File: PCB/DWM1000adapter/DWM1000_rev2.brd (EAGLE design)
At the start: 33.1 x 27.1 mm, 9 parts, among them IC1 DWM1000

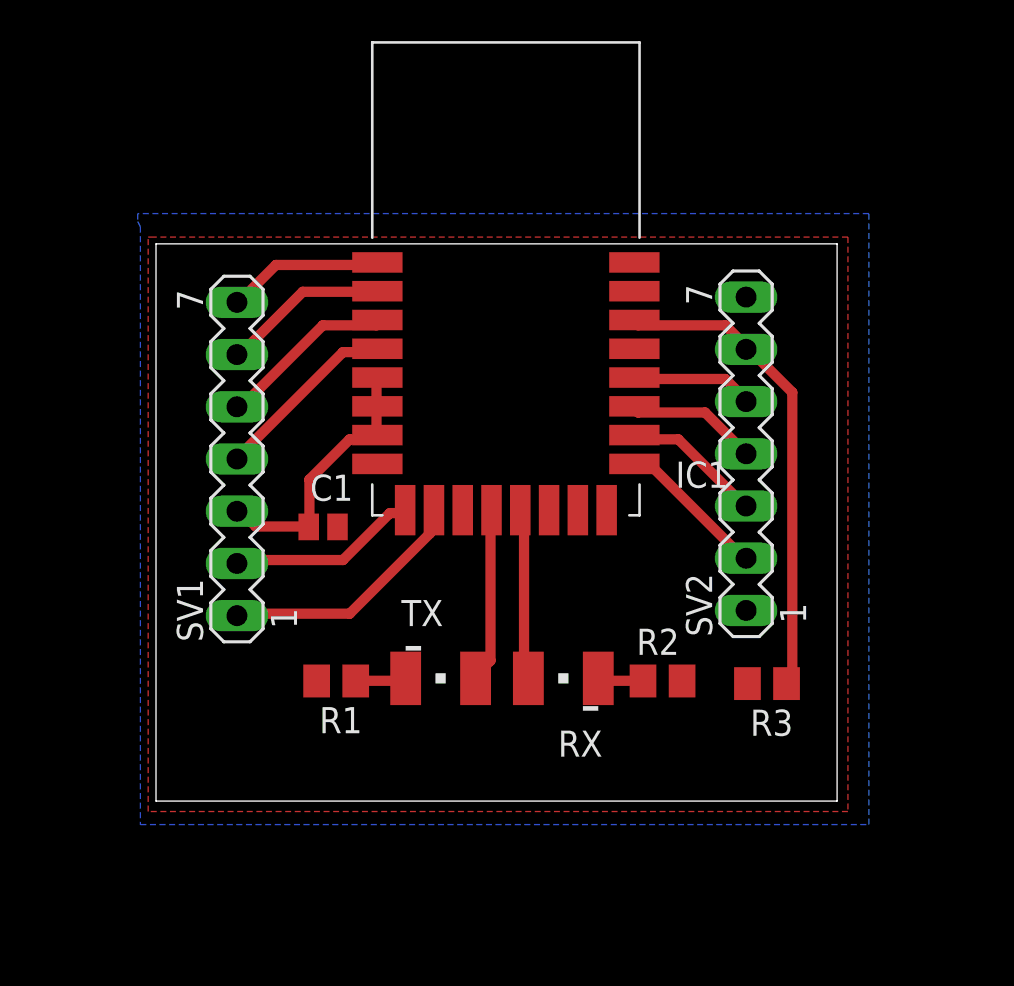
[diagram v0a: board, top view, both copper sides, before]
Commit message: knas
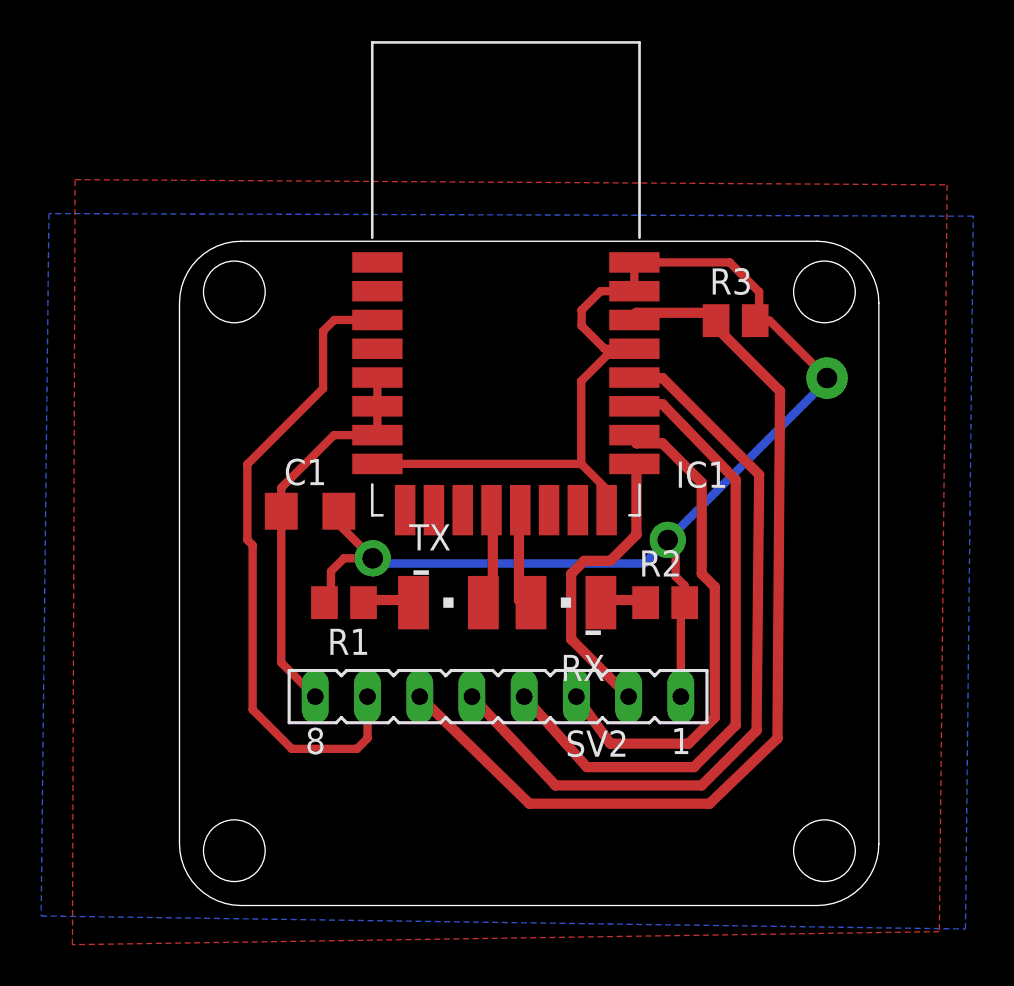
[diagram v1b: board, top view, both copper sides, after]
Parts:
- removed SV1: (no value), con-lstb:MA07-1
- C1: device eagle-ltspice:C0504 -> eagle-ltspice:C1206
- SV2: device con-lstb:MA07-1 -> con-lsta:FE08
- moved R3 17.7 mm to (31.5, 25.0), turned to 0 degrees
- moved SV2 16.9 mm to (19.9, 6.73), turned to 180 degrees
- moved R1 3.83 mm to (12.4, 11.3)
- moved R2 3.81 mm to (28.1, 11.3)
- moved TX 3.70 mm to (17.5, 11.3)
- moved RX 3.69 mm to (23.2, 11.3)
- moved C1 0.99 mm to (10.8, 15.7)
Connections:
- net 3.3: now also SV2.8; no longer SV1.3
- net EXT: no longer SV1.7
- net GND: no longer SV2.7
- net RST: now also SV2.7; no longer SV1.5
- net SPIPHA: no longer SV1.2
- net SPIPOL: no longer SV1.1
- net SYNC: no longer SV1.4
- net WAKE: no longer SV1.6
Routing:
- net GND: track 0.00 -> 82.9 mm, vias 0 -> 3
- net CLK: track 5.94 -> 37.3 mm
- net MISO: track 6.44 -> 31.1 mm
- net IRQ: track 23.6 -> 47.0 mm
- net RST: track 8.68 -> 31.5 mm
- net MOSI: track 6.88 -> 24.5 mm
- net SPIPOL: track 12.2 -> 0.00 mm
- net SPIPHA: track 9.25 -> 0.00 mm
- net SYNC: track 9.12 -> 0.00 mm
- net WAKE: track 8.08 -> 0.00 mm
- net EXT: track 7.65 -> 0.00 mm
- net CS: track 7.42 -> 14.6 mm
- net 3.3: track 13.2 -> 19.4 mm
- net TXLED: track 8.47 -> 4.85 mm
- net RXLED: track 8.36 -> 4.97 mm
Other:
- board size 33.1 x 27.1 mm -> 34 x 32.3 mm
- board text added: "3.3"
- board text added: "CLK"
- board text added: "CS"
- board text added: "GND"
- board text added: "IRQ"
- board text added: "MISO"
- board text added: "MOSI"
- board text added: "Mikael & Filip"
- board text added: "RST"
- board text added: "RX"
- board text added: "TX"
- board text added: "UWB Adapter"
